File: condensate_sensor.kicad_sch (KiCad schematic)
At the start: 4 parts

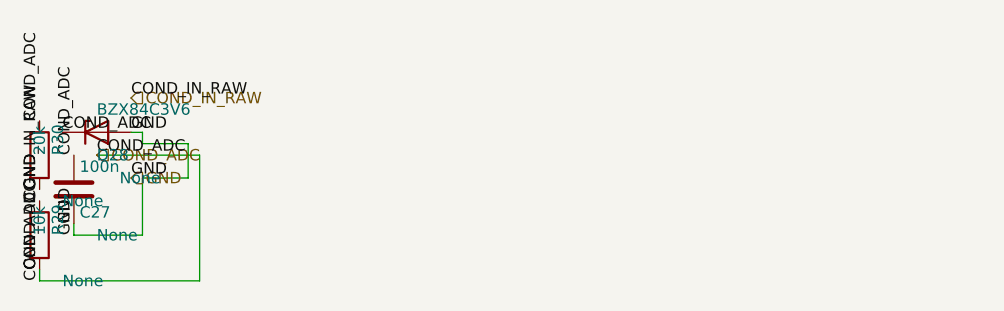
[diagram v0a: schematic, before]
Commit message: tests_fix
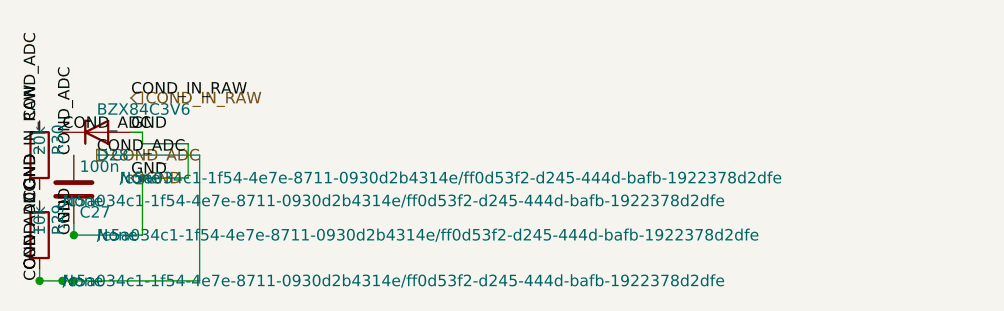
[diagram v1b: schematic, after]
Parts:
- C27, D28, R29, R30: hierarchy_path (none) -> /c5a034c1-1f54-4e7e-8711-0930d2b4314e/ff0d53f2-d245-444d-ba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
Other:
- title: (none) -> climate_control_niva_travel
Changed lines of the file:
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@@
 	(generator_version "9.0")
 	(paper "A4")
+	(title_block
+		(title "climate_control_niva_travel")
+	)
 	(symbol
 		(lib_id "Device:C")
@@
 			)
 		)
+		(property "hierarchy_path" "/c5a034c1-1f54-4e7e-8711-0930d2b4314e/ff0d53f2-d245-444d-bafb-1922378d2dfe"
+			(at 20.32 22.8599 0)
+			(effects
+				(font
+					(size 1.27 1.27)
+				)
+				(justify left)
+			)
+		)
 		(pin "1"
 		)
@@
 		)
 		(instances
-			(project "Untitled"
-				(path "/ccabdeb9-ab3d-40ba-882e-380bf8b75305"
+			(project "climate_control_niva_travel"
+				(path "/c5a034c1-1f54-4e7e-8711-0930d2b4314e/ff0d53f2-d245-444d-bafb-1922378d2dfe"
 					(reference "C27")
 					(unit 1)
@@
 			)
 		)
+		(property "hierarchy_path" "/c5a034c1-1f54-4e7e-8711-0930d2b4314e/ff0d53f2-d245-444d-bafb-1922378d2dfe"
+			(at 16.51 27.9399 0)
+			(effects
+				(font
+					(size 1.27 1.27)
+				)
+				(justify left)
+			)
+		)
 		(pin "1"
 		)
@@
 		)
 		(instances
-			(project "Untitled"
-				(path "/ccabdeb9-ab3d-40ba-882e-380bf8b75305"
+			(project "climate_control_niva_travel"
+				(path "/c5a034c1-1f54-4e7e-8711-0930d2b4314e/ff0d53f2-d245-444d-bafb-1922378d2dfe"
 					(reference "R29")
 					(unit 1)
@@
 			)
 		)
+		(property "hierarchy_path" "/c5a034c1-1f54-4e7e-8711-0930d2b4314e/ff0d53f2-d245-444d-bafb-1922378d2dfe"
+			(at 16.51 19.0499 0)
+			(effects
+				(font
+					(size 1.27 1.27)
+				)
+				(justify left)
+			)
+		)
 		(pin "1"
 		)
@@
 		)
 		(instances
-			(project "Untitled"
-				(path "/ccabdeb9-ab3d-40ba-882e-380bf8b75305"
+			(project "climate_control_niva_travel"
+				(path "/c5a034c1-1f54-4e7e-8711-0930d2b4314e/ff0d53f2-d245-444d-bafb-1922378d2dfe"
 					(reference "R30")
 					(unit 1)
@@
 			)
 		)
+		(property "hierarchy_path" "/c5a034c1-1f54-4e7e-8711-0930d2b4314e/ff0d53f2-d245-444d-bafb-1922378d2dfe"
+			(at 22.86 16.5099 0)
+			(effects
+				(font
+					(size 1.27 1.27)
+				)
+				(justify left)
+			)
+		)
 		(pin "1"
 		)
@@
 		)
 		(instances
-			(project "Untitled"
-				(path "/ccabdeb9-ab3d-40ba-882e-380bf8b75305"
+			(project "climate_control_niva_travel"
+				(path "/c5a034c1-1f54-4e7e-8711-0930d2b4314e/ff0d53f2-d245-444d-bafb-1922378d2dfe"
 					(reference "D28")
 					(unit 1)
@@
 			(type default)
 		)
+	)
+	(junction
+		(at 17.78 22.86)
+		(diameter 0)
+		(color 0 0 0 0)
+	)
+	(junction
+		(at 25.4 16.51)
+		(diameter 0)
+		(color 0 0 0 0)
+	)
+	(junction
+		(at 13.97 27.94)
+		(diameter 0)
+		(color 0 0 0 0)
+	)
+	(junction
+		(at 17.78 27.94)
+		(diameter 0)
+		(color 0 0 0 0)
+	)
+	(junction
+		(at 16.51 27.94)
+		(diameter 0)
+		(color 0 0 0 0)
 	)
 	(label "GND"
@@
 	)
 	(hierarchical_label "COND_ADC"
-		(shape input)
+		(shape output)
 		(at 20.32 13.97 0)
 		(effects

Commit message: refactoring
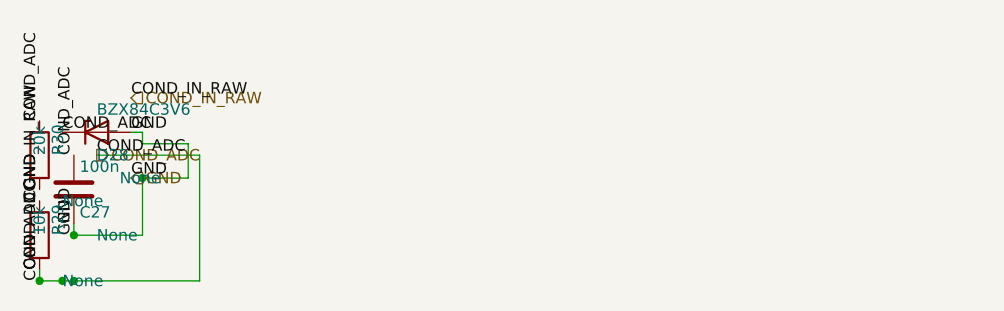
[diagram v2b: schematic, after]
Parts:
- C27, D28, R29, R30: hierarchy_path /c5a034c1-1f54-4e7e-8711-0930d2b4314e/ff0d53f2-d245-444d-ba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 -> (none)
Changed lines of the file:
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@@
-			)
-		)
-		(property "hierarchy_path" "/c5a034c1-1f54-4e7e-8711-0930d2b4314e/ff0d53f2-d245-444d-bafb-1922378d2dfe"
-			(at 20.32 22.8599 0)
-			(effects
-				(font
-					(size 1.27 1.27)
-				)
-				(justify left)
 			)
 		)
@@
 		(instances
 			(project "climate_control_niva_travel"
-				(path "/c5a034c1-1f54-4e7e-8711-0930d2b4314e/ff0d53f2-d245-444d-bafb-1922378d2dfe"
-					(reference "C27")
+				(path "/165a98f1-2dde-4141-9fdc-c935d39c8cff/1b4a3c6f-89c1-46ad-a2ac-968f23f1685b/"
+					(reference "C0627")
 					(unit 1)
 				)
@@
 			)
 		)
-		(property "hierarchy_path" "/c5a034c1-1f54-4e7e-8711-0930d2b4314e/ff0d53f2-d245-444d-bafb-1922378d2dfe"
-			(at 16.51 27.9399 0)
-			(effects
-				(font
-					(size 1.27 1.27)
-				)
-				(justify left)
-			)
-		)
 		(pin "1"
 		)
@@
 		(instances
 			(project "climate_control_niva_travel"
-				(path "/c5a034c1-1f54-4e7e-8711-0930d2b4314e/ff0d53f2-d245-444d-bafb-1922378d2dfe"
-					(reference "R29")
+				(path "/165a98f1-2dde-4141-9fdc-c935d39c8cff/1b4a3c6f-89c1-46ad-a2ac-968f23f1685b/"
+					(reference "R0629")
 					(unit 1)
 				)
@@
 			)
 		)
-		(property "hierarchy_path" "/c5a034c1-1f54-4e7e-8711-0930d2b4314e/ff0d53f2-d245-444d-bafb-1922378d2dfe"
-			(at 16.51 19.0499 0)
-			(effects
-				(font
-					(size 1.27 1.27)
-				)
-				(justify left)
-			)
-		)
 		(pin "1"
 		)
@@
 		(instances
 			(project "climate_control_niva_travel"
-				(path "/c5a034c1-1f54-4e7e-8711-0930d2b4314e/ff0d53f2-d245-444d-bafb-1922378d2dfe"
-					(reference "R30")
+				(path "/165a98f1-2dde-4141-9fdc-c935d39c8cff/1b4a3c6f-89c1-46ad-a2ac-968f23f1685b/"
+					(reference "R0630")
 					(unit 1)
 				)
@@
 			)
 		)
-		(property "hierarchy_path" "/c5a034c1-1f54-4e7e-8711-0930d2b4314e/ff0d53f2-d245-444d-bafb-1922378d2dfe"
-			(at 22.86 16.5099 0)
-			(effects
-				(font
-					(size 1.27 1.27)
-				)
-				(justify left)
-			)
-		)
 		(pin "1"
 		)
@@
 		(instances
 			(project "climate_control_niva_travel"
-				(path "/c5a034c1-1f54-4e7e-8711-0930d2b4314e/ff0d53f2-d245-444d-bafb-1922378d2dfe"
-					(reference "D28")
+				(path "/165a98f1-2dde-4141-9fdc-c935d39c8cff/1b4a3c6f-89c1-46ad-a2ac-968f23f1685b/"
+					(reference "D0628")
 					(unit 1)
 				)

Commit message: refactoring
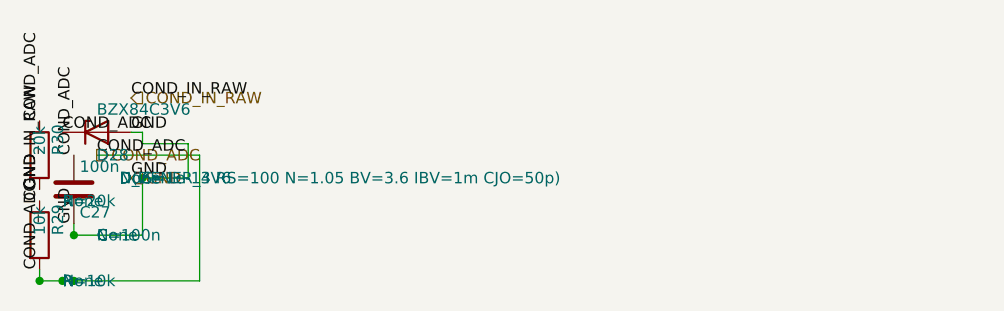
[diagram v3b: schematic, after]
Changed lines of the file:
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@@
+			)
+		)
+		(property "Sim.Device" "C"
+			(at 20.32 22.8599 0)
+			(effects
+				(font
+					(size 1.27 1.27)
+				)
+				(justify left)
+			)
+		)
+		(property "Sim.Params" "C=100n"
+			(at 20.32 22.8599 0)
+			(effects
+				(font
+					(size 1.27 1.27)
+				)
+				(justify left)
 			)
 		)
@@
 		(instances
 			(project "climate_control_niva_travel"
-				(path "/165a98f1-2dde-4141-9fdc-c935d39c8cff/1b4a3c6f-89c1-46ad-a2ac-968f23f1685b/"
+				(path "/cc416b40-1361-4232-ac1e-5cd36ef0c0fb/d17c2923-8318-4f90-a809-98cb9394d6b8/"
 					(reference "C0627")
 					(unit 1)
@@
 			)
 		)
+		(property "Sim.Device" "R"
+			(at 16.51 27.9399 0)
+			(effects
+				(font
+					(size 1.27 1.27)
+				)
+				(justify left)
+			)
+		)
+		(property "Sim.Params" "R=10k"
+			(at 16.51 27.9399 0)
+			(effects
+				(font
+					(size 1.27 1.27)
+				)
+				(justify left)
+			)
+		)
 		(pin "1"
 		)
@@
 		(instances
 			(project "climate_control_niva_travel"
-				(path "/165a98f1-2dde-4141-9fdc-c935d39c8cff/1b4a3c6f-89c1-46ad-a2ac-968f23f1685b/"
+				(path "/cc416b40-1361-4232-ac1e-5cd36ef0c0fb/d17c2923-8318-4f90-a809-98cb9394d6b8/"
 					(reference "R0629")
 					(unit 1)
@@
 			)
 		)
+		(property "Sim.Device" "R"
+			(at 16.51 19.0499 0)
+			(effects
+				(font
+					(size 1.27 1.27)
+				)
+				(justify left)
+			)
+		)
+		(property "Sim.Params" "R=20k"
+			(at 16.51 19.0499 0)
+			(effects
+				(font
+					(size 1.27 1.27)
+				)
+				(justify left)
+			)
+		)
 		(pin "1"
 		)
@@
 		(instances
 			(project "climate_control_niva_travel"
-				(path "/165a98f1-2dde-4141-9fdc-c935d39c8cff/1b4a3c6f-89c1-46ad-a2ac-968f23f1685b/"
+				(path "/cc416b40-1361-4232-ac1e-5cd36ef0c0fb/d17c2923-8318-4f90-a809-98cb9394d6b8/"
 					(reference "R0630")
 					(unit 1)
@@
 			)
 		)
+		(property "Sim.Device" "D"
+			(at 22.86 16.5099 0)
+			(effects
+				(font
+					(size 1.27 1.27)
+				)
+				(justify left)
+			)
+		)
+		(property "Sim.Model" "D_ZENER_3V6"
+			(at 22.86 16.5099 0)
+			(effects
+				(font
+					(size 1.27 1.27)
+				)
+				(justify left)
+			)
+		)
+		(property "Sim.Params" "D(IS=1e-14 RS=100 N=1.05 BV=3.6 IBV=1m CJO=50p)"
+			(at 22.86 16.5099 0)
+			(effects
+				(font
+					(size 1.27 1.27)
+				)
+				(justify left)
+			)
+		)
 		(pin "1"
 		)
@@
 		(instances
 			(project "climate_control_niva_travel"
-				(path "/165a98f1-2dde-4141-9fdc-c935d39c8cff/1b4a3c6f-89c1-46ad-a2ac-968f23f1685b/"
+				(path "/cc416b40-1361-4232-ac1e-5cd36ef0c0fb/d17c2923-8318-4f90-a809-98cb9394d6b8/"
 					(reference "D0628")
 					(unit 1)
@@
 	(junction
 		(at 17.78 22.86)
-		(diameter 0)
+		(diameter 0.0000)
 		(color 0 0 0 0)
 	)
 	(junction
 		(at 25.4 16.51)
-		(diameter 0)
+		(diameter 0.0000)
 		(color 0 0 0 0)
 	)
 	(junction
 		(at 13.97 27.94)
-		(diameter 0)
+		(diameter 0.0000)
 		(color 0 0 0 0)
 	)
 	(junction
 		(at 17.78 27.94)
-		(diameter 0)
+		(diameter 0.0000)
 		(color 0 0 0 0)
 	)
 	(junction
 		(at 16.51 27.94)
-		(diameter 0)
+		(diameter 0.0000)
 		(color 0 0 0 0)
 	)
@@
 		)
 	)
-	(label "GND"
-		(at 17.78 22.86 270)
-		(effects
-			(font
-				(size 1.27 1.27)
-			)
-			(justify left bottom)
-		)
-	)
 	(label "COND_IN_RAW"
 		(at 13.97 19.05 90)
@@
 		(effects
 			(font
-				(size 1.27 1.27)
-			)
-			(justify left bottom)
-		)
-	)
-	(label "COND_ADC"
-		(at 13.97 27.94 90)
-		(effects
-			(font
